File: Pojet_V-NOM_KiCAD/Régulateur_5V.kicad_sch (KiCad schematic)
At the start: 30 parts, among them IC1001 MP1475SGJ-P, IC1002 MP1475SGJ-P

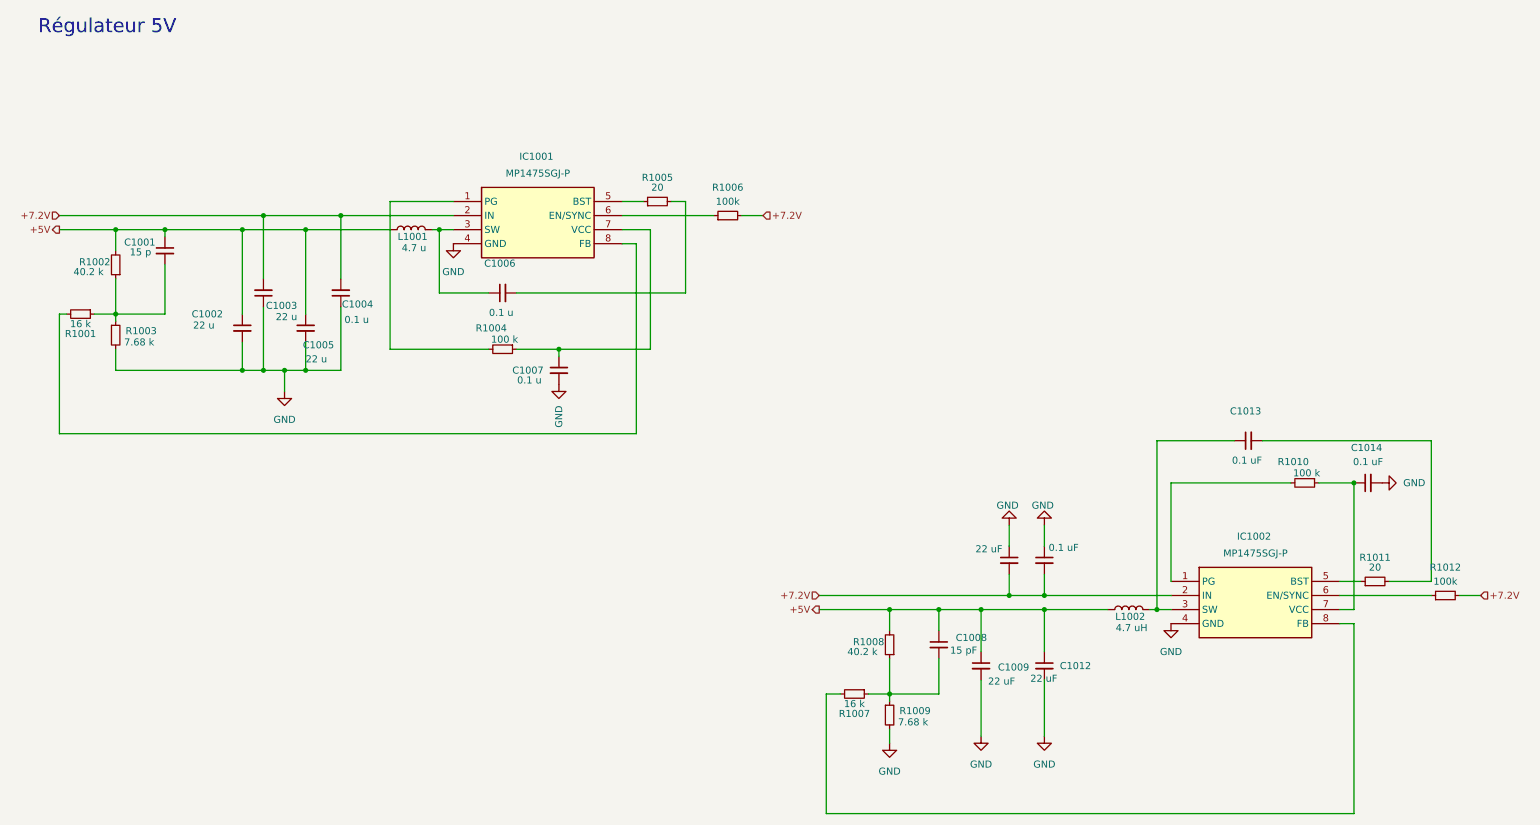
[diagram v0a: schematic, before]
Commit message: maj regulateur 5V
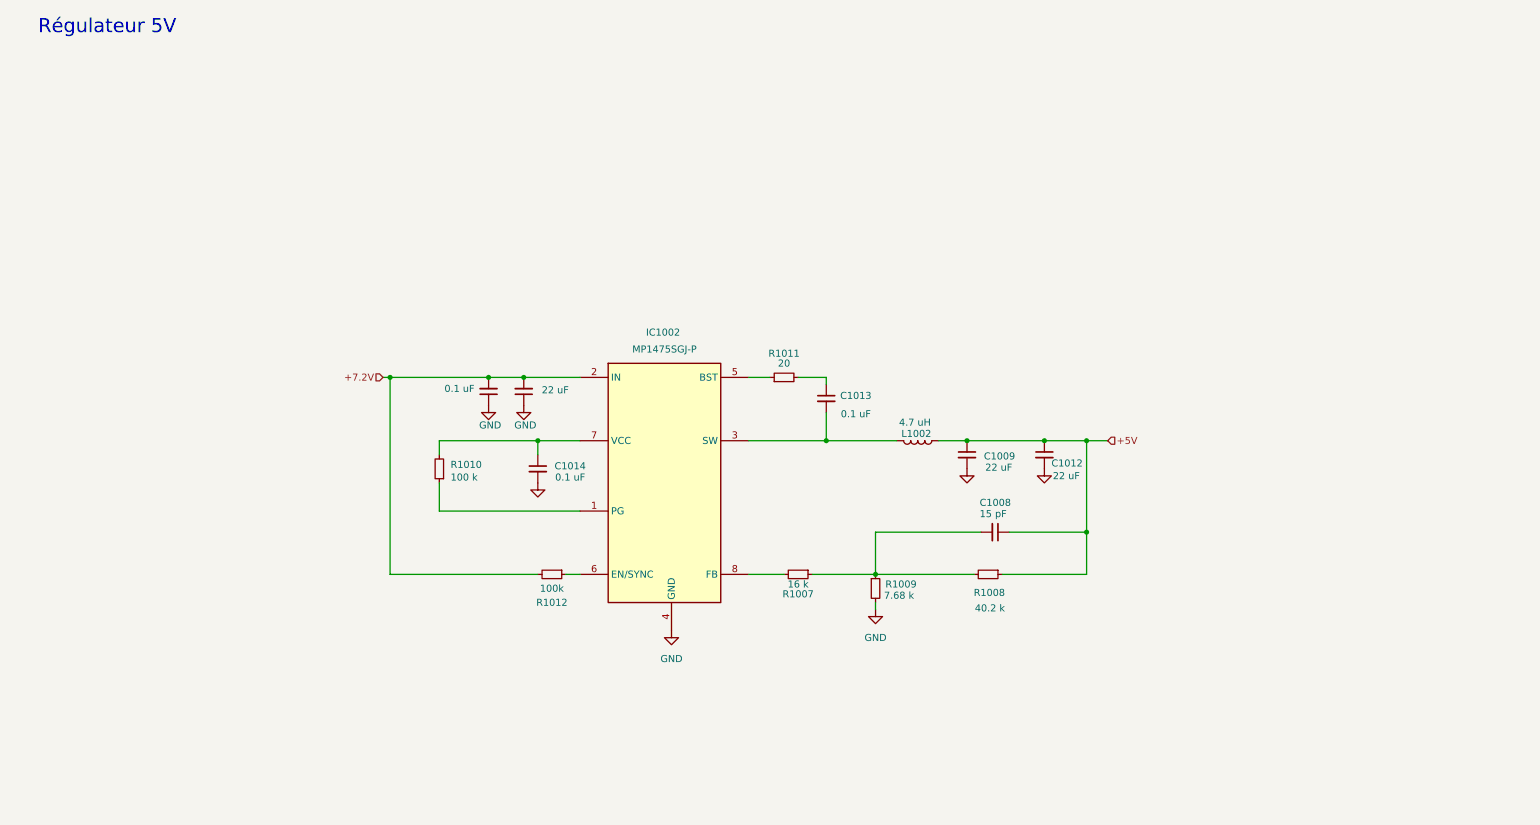
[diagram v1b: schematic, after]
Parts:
- removed C1001: 15 p, symbol Device:C_Small
- removed C1002, C1003, C1005: 22 u, symbol Device:C_Small
- removed C1004, C1006, C1007: 0.1 u, symbol Device:C_Small
- removed IC1001: MP1475SGJ-P, SOT65P280X100-8N, symbol MP1475SGJ-P:MP1475SGJ-P
- removed L1001: 4.7 u, symbol Device:L
- removed R1001: 16 k, symbol Device:R_Small
- removed R1002: 40.2 k, symbol Device:R_Small
- removed R1003: 7.68 k, symbol Device:R_Small
- removed R1004: 100 k, symbol Device:R_Small
- removed R1005: 20, symbol Device:R_Small
- removed R1006: 100k, symbol Device:R_Small
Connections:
- net +5V: now also R1008.1; no longer R1008.2
- net at R1011.2: now also C1013.1; no longer C1013.2
- net at C1008.2, R1007.1, R1009.1: now also R1008.2; no longer R1008.1
- net at IC1002.3 (SW), L1002.2: now also C1013.2; no longer C1013.1
- net at C1014.1, IC1002.7 (VCC): now also R1010.2; no longer R1010.1
- net at IC1002.1 (PG): now also R1010.1; no longer R1010.2
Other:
- moved on the sheet: C1008, C1009, C1012, C1013, C1014, IC1002, L1002, R1007, R1008, R1009, R1010, R1011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
